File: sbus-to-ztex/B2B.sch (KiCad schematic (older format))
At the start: 6 parts, among them J1 Conn_01x06_Male, J3 Conn_02x07_Odd_Even

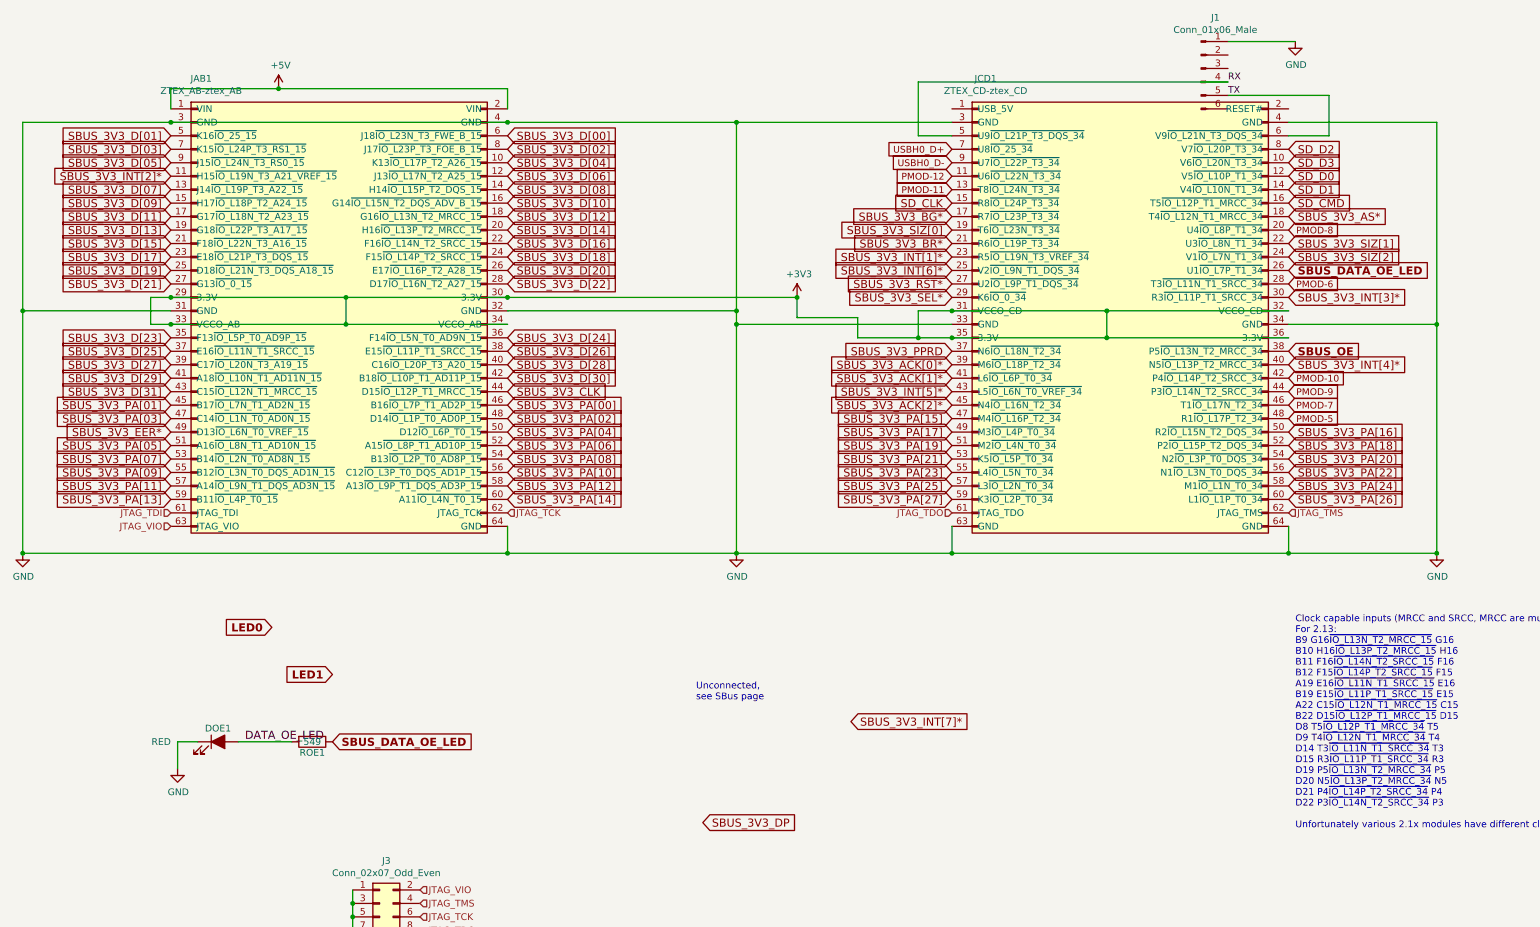
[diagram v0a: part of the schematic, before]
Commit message: thinking about a V1.3
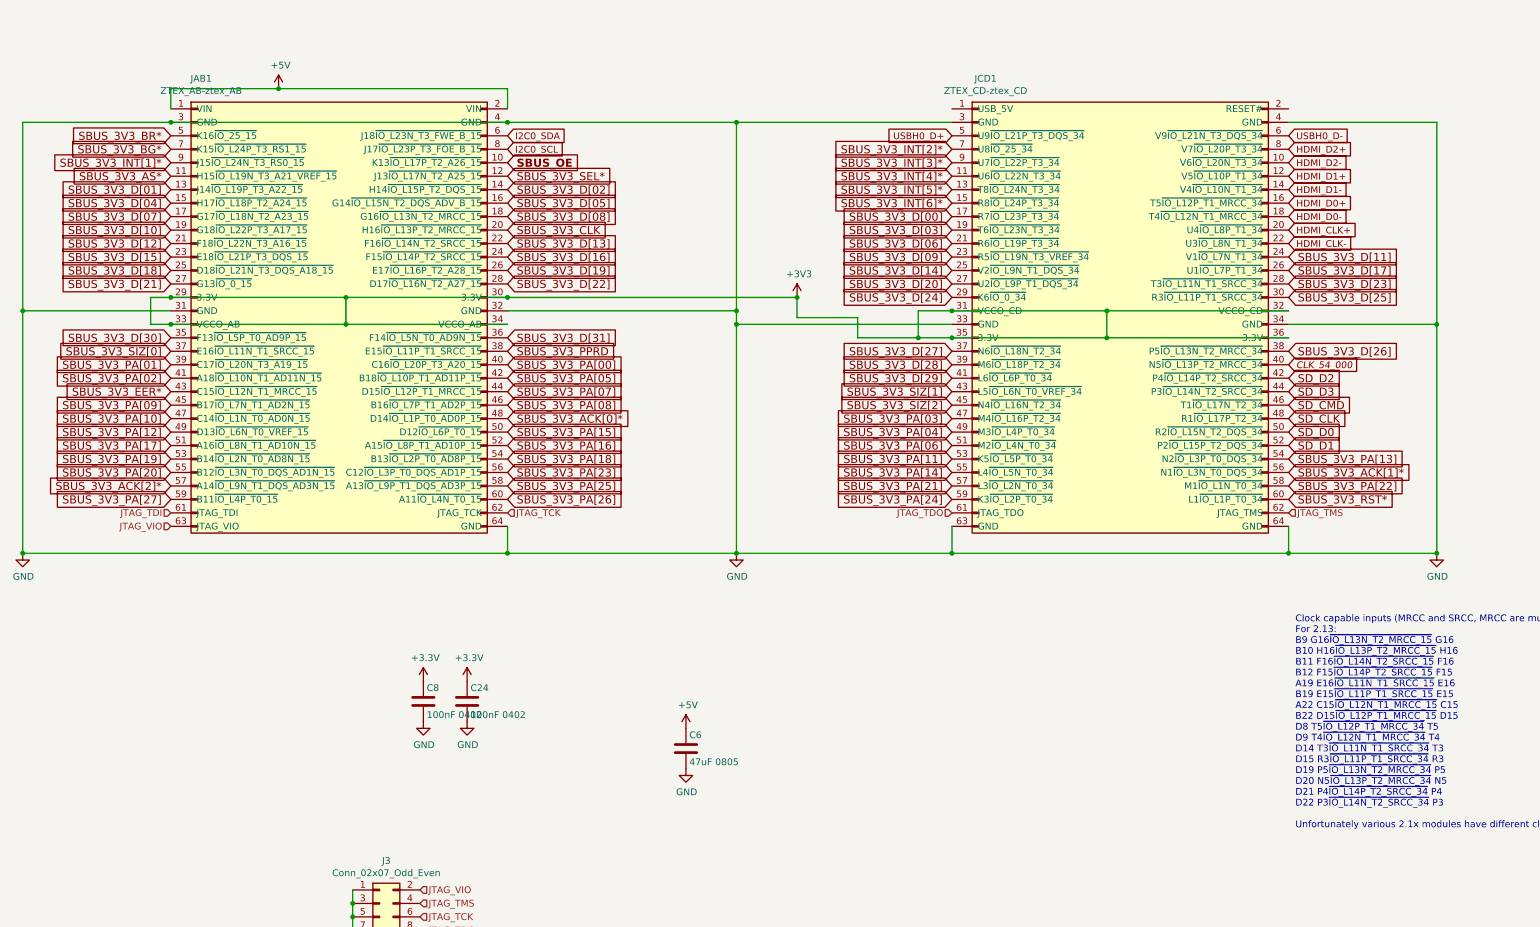
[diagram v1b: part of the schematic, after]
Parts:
- removed DOE1: RED, LED_SMD:LED_0805_2012Metric, symbol Device:LED_ALT
- removed J1: Conn_01x06_Male, For_SeeedStudio:PinHeader_1x06_P2.54mm_Horizontal_For_SeeedStudio, symbol Connector:Conn_01x06_Male
- removed ROE1: 549, Resistor_SMD:R_0603_1608Metric, symbol Device:R
- added C24, C8: 100nF 0402, Capacitor_SMD:C_0402_1005Metric, symbol Device:C
- added C6: 47uF 0805, Capacitor_SMD:C_0805_2012Metric, symbol Device:C
- J3: DNP (none) -> DNP
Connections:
- net PMOD-10 is gone; now on net SD_D2: JCD1.42 (P4~IO_L14P_T2_SRCC_34)
- net PMOD-11 is gone; now on net SBUS_3V3_INT[5]*: JCD1.13 (T8~IO_L24N_T3_34)
- net PMOD-12 is gone; now on net SBUS_3V3_INT[4]*: JCD1.11 (U6~IO_L22N_T3_34)
- net PMOD-5 is gone; now on net SD_CLK: JCD1.48 (R1~IO_L17P_T2_34)
- net PMOD-6 is gone; now on net SBUS_3V3_D[23]: JCD1.28 (T3~IO_L11N_T1_SRCC_34)
- net PMOD-7 is gone; now on net SD_CMD: JCD1.46 (T1~IO_L17N_T2_34)
- net PMOD-9 is gone; now on net SD_D3: JCD1.44 (P3~IO_L14N_T2_SRCC_34)
- net RX is gone; now on net USBH0_D+: JCD1.5 (U9~IO_L21P_T3_DQS_34)
- net SBUS_DATA_OE_LED is gone; now on net SBUS_3V3_D[17]: JCD1.26 (U1~IO_L7P_T1_34)
- net TX is gone; now on net USBH0_D-: JCD1.6 (V9~IO_L21N_T3_DQS_34)
- net +3V3: now also C24.1, C8.1
- net +5V: now also C6.1
- net GND: now also C24.2, C6.2, C8.2
- net SBUS_3V3_ACK[0]*: now also JAB1.48 (D14~IO_L1P_T0_AD0P_15); no longer JCD1.39 (M6~IO_L18P_T2_34)
- net SBUS_3V3_ACK[1]*: now also JCD1.56 (N1~IO_L3N_T0_DQS_34); no longer JCD1.41 (L6~IO_L6P_T0_34)
- net SBUS_3V3_ACK[2]*: now also JAB1.57 (A14~IO_L9N_T1_DQS_AD3N_15); no longer JCD1.45 (N4~IO_L16N_T2_34)
- net SBUS_3V3_AS*: now also JAB1.11 (H15~IO_L19N_T3_A21_VREF_15); no longer JCD1.18 (T4~IO_L12N_T1_MRCC_34)
- net SBUS_3V3_BG*: now also JAB1.7 (K15~IO_L24P_T3_RS1_15); no longer JCD1.17 (R7~IO_L23P_T3_34)
- net SBUS_3V3_BR*: now also JAB1.5 (K16~IO_25_15); no longer JCD1.21 (R6~IO_L19P_T3_34)
- net SBUS_3V3_CLK: now also JAB1.20 (H16~IO_L13P_T2_MRCC_15); no longer JAB1.44 (D15~IO_L12P_T1_MRCC_15)
- net SBUS_3V3_D[00]: now also JCD1.17 (R7~IO_L23P_T3_34); no longer JAB1.6 (J18~IO_L23N_T3_FWE_B_15)
- net SBUS_3V3_D[01]: now also JAB1.13 (J14~IO_L19P_T3_A22_15); no longer JAB1.5 (K16~IO_25_15)
- net SBUS_3V3_D[02]: now also JAB1.14 (H14~IO_L15P_T2_DQS_15); no longer JAB1.8 (J17~IO_L23P_T3_FOE_B_15)
- net SBUS_3V3_D[03]: now also JCD1.19 (T6~IO_L23N_T3_34); no longer JAB1.7 (K15~IO_L24P_T3_RS1_15)
- net SBUS_3V3_D[04]: now also JAB1.15 (H17~IO_L18P_T2_A24_15); no longer JAB1.10 (K13~IO_L17P_T2_A26_15)
- net SBUS_3V3_D[05]: now also JAB1.16 (G14~IO_L15N_T2_DQS_ADV_B_15); no longer JAB1.9 (J15~IO_L24N_T3_RS0_15)
- net SBUS_3V3_D[06]: now also JCD1.21 (R6~IO_L19P_T3_34); no longer JAB1.12 (J13~IO_L17N_T2_A25_15)
- net SBUS_3V3_D[07]: now also JAB1.17 (G17~IO_L18N_T2_A23_15); no longer JAB1.13 (J14~IO_L19P_T3_A22_15)
- net SBUS_3V3_D[08]: now also JAB1.18 (G16~IO_L13N_T2_MRCC_15); no longer JAB1.14 (H14~IO_L15P_T2_DQS_15)
- net SBUS_3V3_D[09]: now also JCD1.23 (R5~IO_L19N_T3_VREF_34); no longer JAB1.15 (H17~IO_L18P_T2_A24_15)
- net SBUS_3V3_D[10]: now also JAB1.19 (G18~IO_L22P_T3_A17_15); no longer JAB1.16 (G14~IO_L15N_T2_DQS_ADV_B_15)
- net SBUS_3V3_D[11]: now also JCD1.24 (V1~IO_L7N_T1_34); no longer JAB1.17 (G17~IO_L18N_T2_A23_15)
- net SBUS_3V3_D[12]: now also JAB1.21 (F18~IO_L22N_T3_A16_15); no longer JAB1.18 (G16~IO_L13N_T2_MRCC_15)
- net SBUS_3V3_D[13]: now also JAB1.22 (F16~IO_L14N_T2_SRCC_15); no longer JAB1.19 (G18~IO_L22P_T3_A17_15)
- net SBUS_3V3_D[14]: now also JCD1.25 (V2~IO_L9N_T1_DQS_34); no longer JAB1.20 (H16~IO_L13P_T2_MRCC_15)
- net SBUS_3V3_D[15]: now also JAB1.23 (E18~IO_L21P_T3_DQS_15); no longer JAB1.21 (F18~IO_L22N_T3_A16_15)
- net SBUS_3V3_D[16]: now also JAB1.24 (F15~IO_L14P_T2_SRCC_15); no longer JAB1.22 (F16~IO_L14N_T2_SRCC_15)
- net SBUS_3V3_D[17]: no longer JAB1.23 (E18~IO_L21P_T3_DQS_15)
- net SBUS_3V3_D[18]: now also JAB1.25 (D18~IO_L21N_T3_DQS_A18_15); no longer JAB1.24 (F15~IO_L14P_T2_SRCC_15)
- net SBUS_3V3_D[19]: now also JAB1.26 (E17~IO_L16P_T2_A28_15); no longer JAB1.25 (D18~IO_L21N_T3_DQS_A18_15)
- net SBUS_3V3_D[20]: now also JCD1.27 (U2~IO_L9P_T1_DQS_34); no longer JAB1.26 (E17~IO_L16P_T2_A28_15)
- net SBUS_3V3_D[23]: no longer JAB1.35 (F13~IO_L5P_T0_AD9P_15)
- net SBUS_3V3_D[24]: now also JCD1.29 (K6~IO_0_34); no longer JAB1.36 (F14~IO_L5N_T0_AD9N_15)
- net SBUS_3V3_D[25]: now also JCD1.30 (R3~IO_L11P_T1_SRCC_34); no longer JAB1.37 (E16~IO_L11N_T1_SRCC_15)
- net SBUS_3V3_D[26]: now also JCD1.38 (P5~IO_L13N_T2_MRCC_34); no longer JAB1.38 (E15~IO_L11P_T1_SRCC_15)
- net SBUS_3V3_D[27]: now also JCD1.37 (N6~IO_L18N_T2_34); no longer JAB1.39 (C17~IO_L20N_T3_A19_15)
- net SBUS_3V3_D[28]: now also JCD1.39 (M6~IO_L18P_T2_34); no longer JAB1.40 (C16~IO_L20P_T3_A20_15)
- net SBUS_3V3_D[29]: now also JCD1.41 (L6~IO_L6P_T0_34); no longer JAB1.41 (A18~IO_L10N_T1_AD11N_15)
- net SBUS_3V3_D[30]: now also JAB1.35 (F13~IO_L5P_T0_AD9P_15); no longer JAB1.42 (B18~IO_L10P_T1_AD11P_15)
- net SBUS_3V3_D[31]: now also JAB1.36 (F14~IO_L5N_T0_AD9N_15); no longer JAB1.43 (C15~IO_L12N_T1_MRCC_15)
- net SBUS_3V3_EER*: now also JAB1.43 (C15~IO_L12N_T1_MRCC_15); no longer JAB1.49 (D13~IO_L6N_T0_VREF_15)
- net SBUS_3V3_INT[1]*: now also JAB1.9 (J15~IO_L24N_T3_RS0_15); no longer JCD1.23 (R5~IO_L19N_T3_VREF_34)
- net SBUS_3V3_INT[2]*: now also JCD1.7 (U8~IO_25_34); no longer JAB1.11 (H15~IO_L19N_T3_A21_VREF_15)
- net SBUS_3V3_INT[3]*: now also JCD1.9 (U7~IO_L22P_T3_34); no longer JCD1.30 (R3~IO_L11P_T1_SRCC_34)
- net SBUS_3V3_INT[4]*: no longer JCD1.40 (N5~IO_L13P_T2_MRCC_34)
- net SBUS_3V3_INT[5]*: no longer JCD1.43 (L5~IO_L6N_T0_VREF_34)
- net SBUS_3V3_INT[6]*: now also JCD1.15 (R8~IO_L24P_T3_34); no longer JCD1.25 (V2~IO_L9N_T1_DQS_34)
- net SBUS_3V3_PA[00]: now also JAB1.40 (C16~IO_L20P_T3_A20_15); no longer JAB1.46 (B16~IO_L7P_T1_AD2P_15)
- net SBUS_3V3_PA[01]: now also JAB1.39 (C17~IO_L20N_T3_A19_15); no longer JAB1.45 (B17~IO_L7N_T1_AD2N_15)
- net SBUS_3V3_PA[02]: now also JAB1.41 (A18~IO_L10N_T1_AD11N_15); no longer JAB1.48 (D14~IO_L1P_T0_AD0P_15)
- net SBUS_3V3_PA[03]: now also JCD1.47 (M4~IO_L16P_T2_34); no longer JAB1.47 (C14~IO_L1N_T0_AD0N_15)
- net SBUS_3V3_PA[04]: now also JCD1.49 (M3~IO_L4P_T0_34); no longer JAB1.50 (D12~IO_L6P_T0_15)
- net SBUS_3V3_PA[05]: now also JAB1.42 (B18~IO_L10P_T1_AD11P_15); no longer JAB1.51 (A16~IO_L8N_T1_AD10N_15)
- net SBUS_3V3_PA[06]: now also JCD1.51 (M2~IO_L4N_T0_34); no longer JAB1.52 (A15~IO_L8P_T1_AD10P_15)
- net SBUS_3V3_PA[07]: now also JAB1.44 (D15~IO_L12P_T1_MRCC_15); no longer JAB1.53 (B14~IO_L2N_T0_AD8N_15)
- net SBUS_3V3_PA[08]: now also JAB1.46 (B16~IO_L7P_T1_AD2P_15); no longer JAB1.54 (B13~IO_L2P_T0_AD8P_15)
- net SBUS_3V3_PA[09]: now also JAB1.45 (B17~IO_L7N_T1_AD2N_15); no longer JAB1.55 (B12~IO_L3N_T0_DQS_AD1N_15)
- net SBUS_3V3_PA[10]: now also JAB1.47 (C14~IO_L1N_T0_AD0N_15); no longer JAB1.56 (C12~IO_L3P_T0_DQS_AD1P_15)
- net SBUS_3V3_PA[11]: now also JCD1.53 (K5~IO_L5P_T0_34); no longer JAB1.57 (A14~IO_L9N_T1_DQS_AD3N_15)
- net SBUS_3V3_PA[12]: now also JAB1.49 (D13~IO_L6N_T0_VREF_15); no longer JAB1.58 (A13~IO_L9P_T1_DQS_AD3P_15)
- net SBUS_3V3_PA[13]: now also JCD1.54 (N2~IO_L3P_T0_DQS_34); no longer JAB1.59 (B11~IO_L4P_T0_15)
- net SBUS_3V3_PA[14]: now also JCD1.55 (L4~IO_L5N_T0_34); no longer JAB1.60 (A11~IO_L4N_T0_15)
- net SBUS_3V3_PA[15]: now also JAB1.50 (D12~IO_L6P_T0_15); no longer JCD1.47 (M4~IO_L16P_T2_34)
- net SBUS_3V3_PA[16]: now also JAB1.52 (A15~IO_L8P_T1_AD10P_15); no longer JCD1.50 (R2~IO_L15N_T2_DQS_34)
- net SBUS_3V3_PA[17]: now also JAB1.51 (A16~IO_L8N_T1_AD10N_15); no longer JCD1.49 (M3~IO_L4P_T0_34)
- net SBUS_3V3_PA[18]: now also JAB1.54 (B13~IO_L2P_T0_AD8P_15); no longer JCD1.52 (P2~IO_L15P_T2_DQS_34)
- net SBUS_3V3_PA[19]: now also JAB1.53 (B14~IO_L2N_T0_AD8N_15); no longer JCD1.51 (M2~IO_L4N_T0_34)
- net SBUS_3V3_PA[20]: now also JAB1.55 (B12~IO_L3N_T0_DQS_AD1N_15); no longer JCD1.54 (N2~IO_L3P_T0_DQS_34)
- net SBUS_3V3_PA[21]: now also JCD1.57 (L3~IO_L2N_T0_34); no longer JCD1.53 (K5~IO_L5P_T0_34)
- net SBUS_3V3_PA[22]: now also JCD1.58 (M1~IO_L1N_T0_34); no longer JCD1.56 (N1~IO_L3N_T0_DQS_34)
- net SBUS_3V3_PA[23]: now also JAB1.56 (C12~IO_L3P_T0_DQS_AD1P_15); no longer JCD1.55 (L4~IO_L5N_T0_34)
- net SBUS_3V3_PA[24]: now also JCD1.59 (K3~IO_L2P_T0_34); no longer JCD1.58 (M1~IO_L1N_T0_34)
- net SBUS_3V3_PA[25]: now also JAB1.58 (A13~IO_L9P_T1_DQS_AD3P_15); no longer JCD1.57 (L3~IO_L2N_T0_34)
- net SBUS_3V3_PA[26]: now also JAB1.60 (A11~IO_L4N_T0_15); no longer JCD1.60 (L1~IO_L1P_T0_34)
- net SBUS_3V3_PA[27]: now also JAB1.59 (B11~IO_L4P_T0_15); no longer JCD1.59 (K3~IO_L2P_T0_34)
- net SBUS_3V3_PPRD: now also JAB1.38 (E15~IO_L11P_T1_SRCC_15); no longer JCD1.37 (N6~IO_L18N_T2_34)
- net SBUS_3V3_RST*: now also JCD1.60 (L1~IO_L1P_T0_34); no longer JCD1.27 (U2~IO_L9P_T1_DQS_34)
- net SBUS_3V3_SEL*: now also JAB1.12 (J13~IO_L17N_T2_A25_15); no longer JCD1.29 (K6~IO_0_34)
- net SBUS_3V3_SIZ[0]: now also JAB1.37 (E16~IO_L11N_T1_SRCC_15); no longer JCD1.19 (T6~IO_L23N_T3_34)
- net SBUS_3V3_SIZ[1]: now also JCD1.43 (L5~IO_L6N_T0_VREF_34); no longer JCD1.22 (U3~IO_L8N_T1_34)
- net SBUS_3V3_SIZ[2]: now also JCD1.45 (N4~IO_L16N_T2_34); no longer JCD1.24 (V1~IO_L7N_T1_34)
- net SBUS_OE: now also JAB1.10 (K13~IO_L17P_T2_A26_15); no longer JCD1.38 (P5~IO_L13N_T2_MRCC_34)
- net SD_CLK: no longer JCD1.15 (R8~IO_L24P_T3_34)
- net SD_CMD: no longer JCD1.16 (T5~IO_L12P_T1_MRCC_34)
- net SD_D0: now also JCD1.50 (R2~IO_L15N_T2_DQS_34); no longer JCD1.12 (V5~IO_L10P_T1_34)
- net SD_D1: now also JCD1.52 (P2~IO_L15P_T2_DQS_34); no longer JCD1.14 (V4~IO_L10N_T1_34)
- net SD_D2: no longer JCD1.8 (V7~IO_L20P_T3_34)
- net SD_D3: no longer JCD1.10 (V6~IO_L20N_T3_34)
- net USBH0_D+: no longer JCD1.7 (U8~IO_25_34)
- net USBH0_D-: no longer JCD1.9 (U7~IO_L22P_T3_34)
- net PMOD-8 renamed HDMI_CLK+
- new net CLK_54_000: JCD1.40 (N5~IO_L13P_T2_MRCC_34)
- new net HDMI_CLK-: JCD1.22 (U3~IO_L8N_T1_34)
- new net HDMI_D0+: JCD1.16 (T5~IO_L12P_T1_MRCC_34)
- new net HDMI_D0-: JCD1.18 (T4~IO_L12N_T1_MRCC_34)
- new net HDMI_D1+: JCD1.12 (V5~IO_L10P_T1_34)
- new net HDMI_D1-: JCD1.14 (V4~IO_L10N_T1_34)
- new net HDMI_D2+: JCD1.8 (V7~IO_L20P_T3_34)
- new net HDMI_D2-: JCD1.10 (V6~IO_L20N_T3_34)
- new net I2C0_SCL: JAB1.8 (J17~IO_L23P_T3_FOE_B_15)
- new net I2C0_SDA: JAB1.6 (J18~IO_L23N_T3_FWE_B_15)
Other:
- note removed: "Unconnected,\nsee SBus page"
